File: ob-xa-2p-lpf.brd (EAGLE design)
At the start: 50.8 x 88.9 mm, 53 parts, among them IC1 AS3320, IC3 TL082P

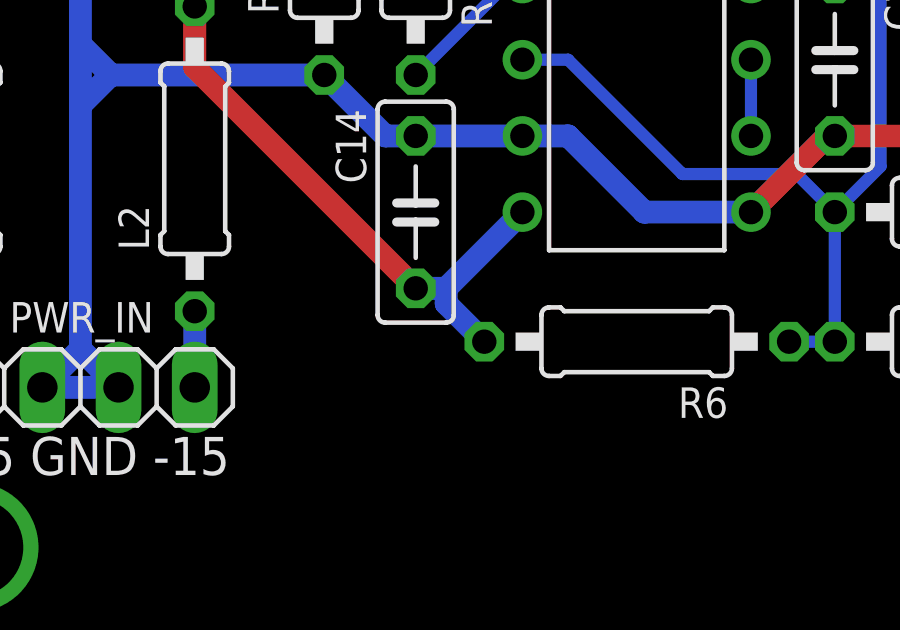
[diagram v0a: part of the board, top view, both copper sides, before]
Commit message: minor cleanup. Draft2 rev
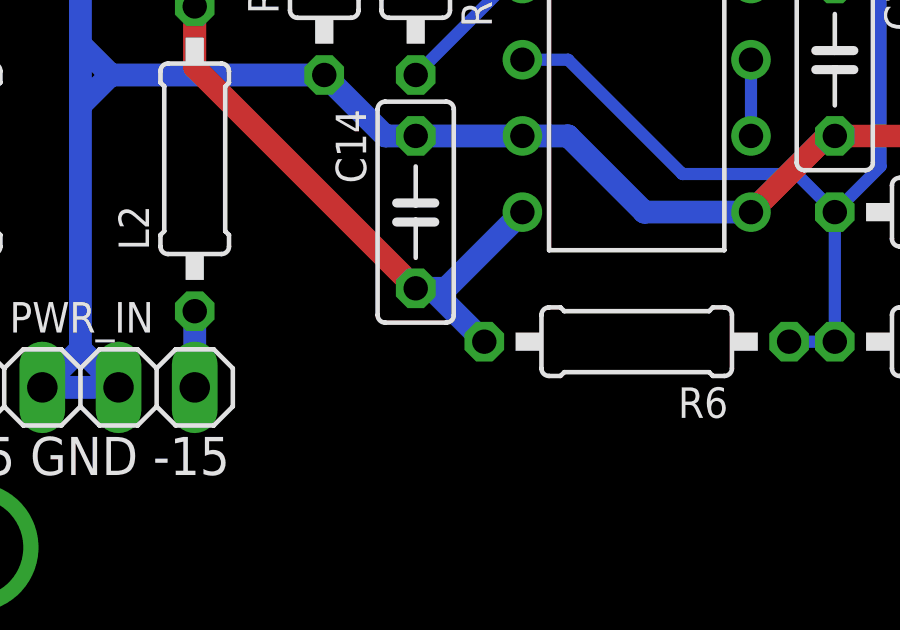
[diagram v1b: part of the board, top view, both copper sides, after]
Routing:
- net -15V: track 66.5 -> 67.2 mm
